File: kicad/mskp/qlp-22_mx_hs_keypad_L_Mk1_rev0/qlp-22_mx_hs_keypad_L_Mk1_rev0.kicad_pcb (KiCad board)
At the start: 2 copper layers, 175.4 x 84.9 mm, 28 parts, among them J1 Conn_01x12_Socket, SW0 Switch, SW1 Switch, SW10 Switch, SW2 Switch, SW3 Switch, SW4 Switch, SW5 Switch, SW6 Switch, SW7 Switch, SW8 Switch, SW9 Switch

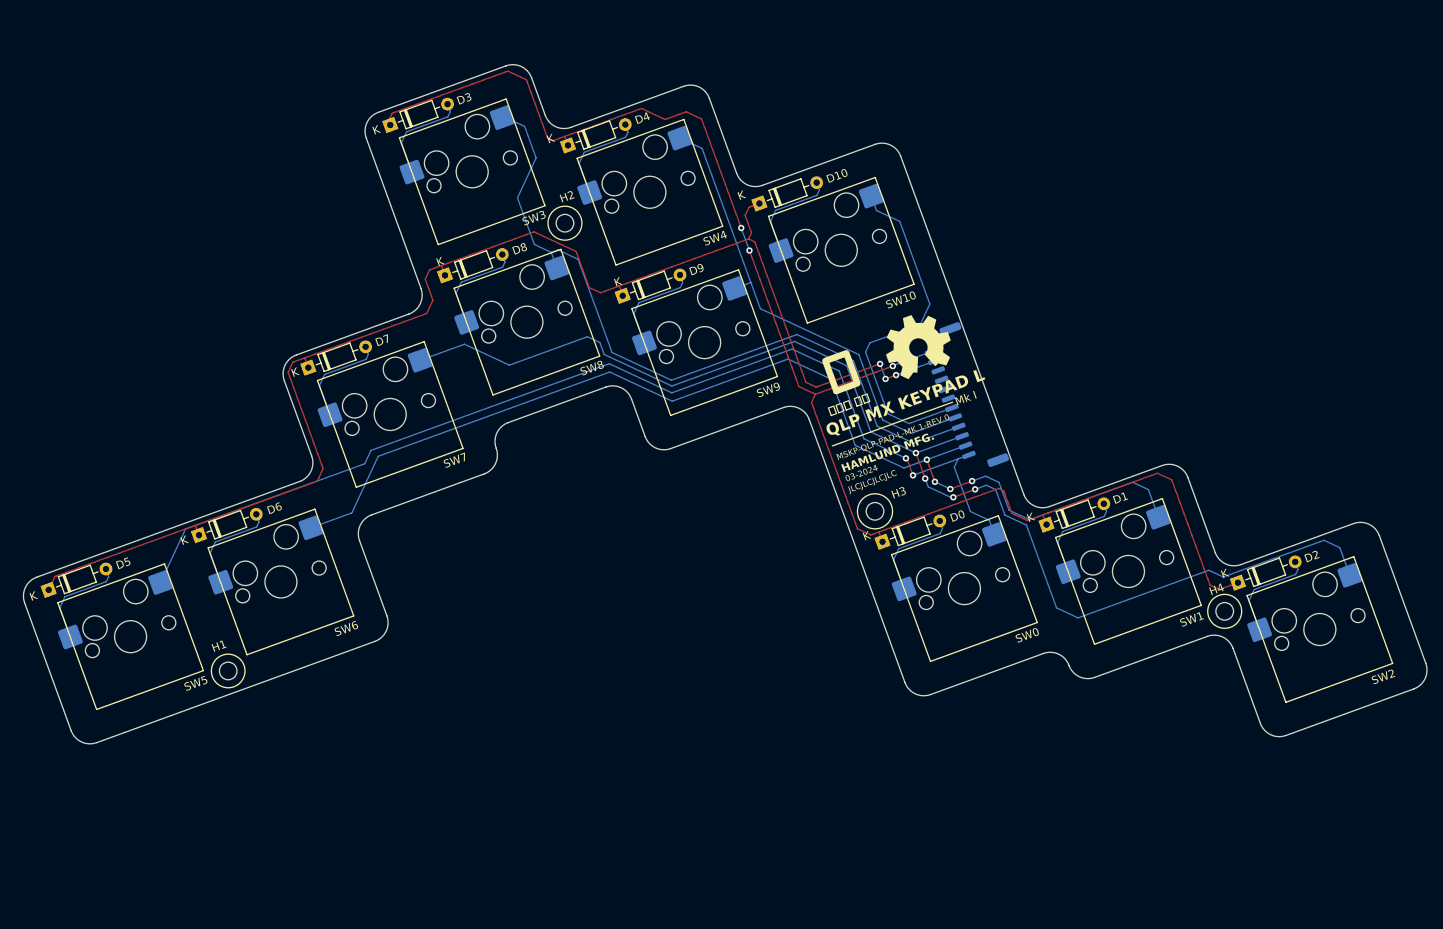
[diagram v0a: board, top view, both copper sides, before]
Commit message: Minor keypad design update ideas
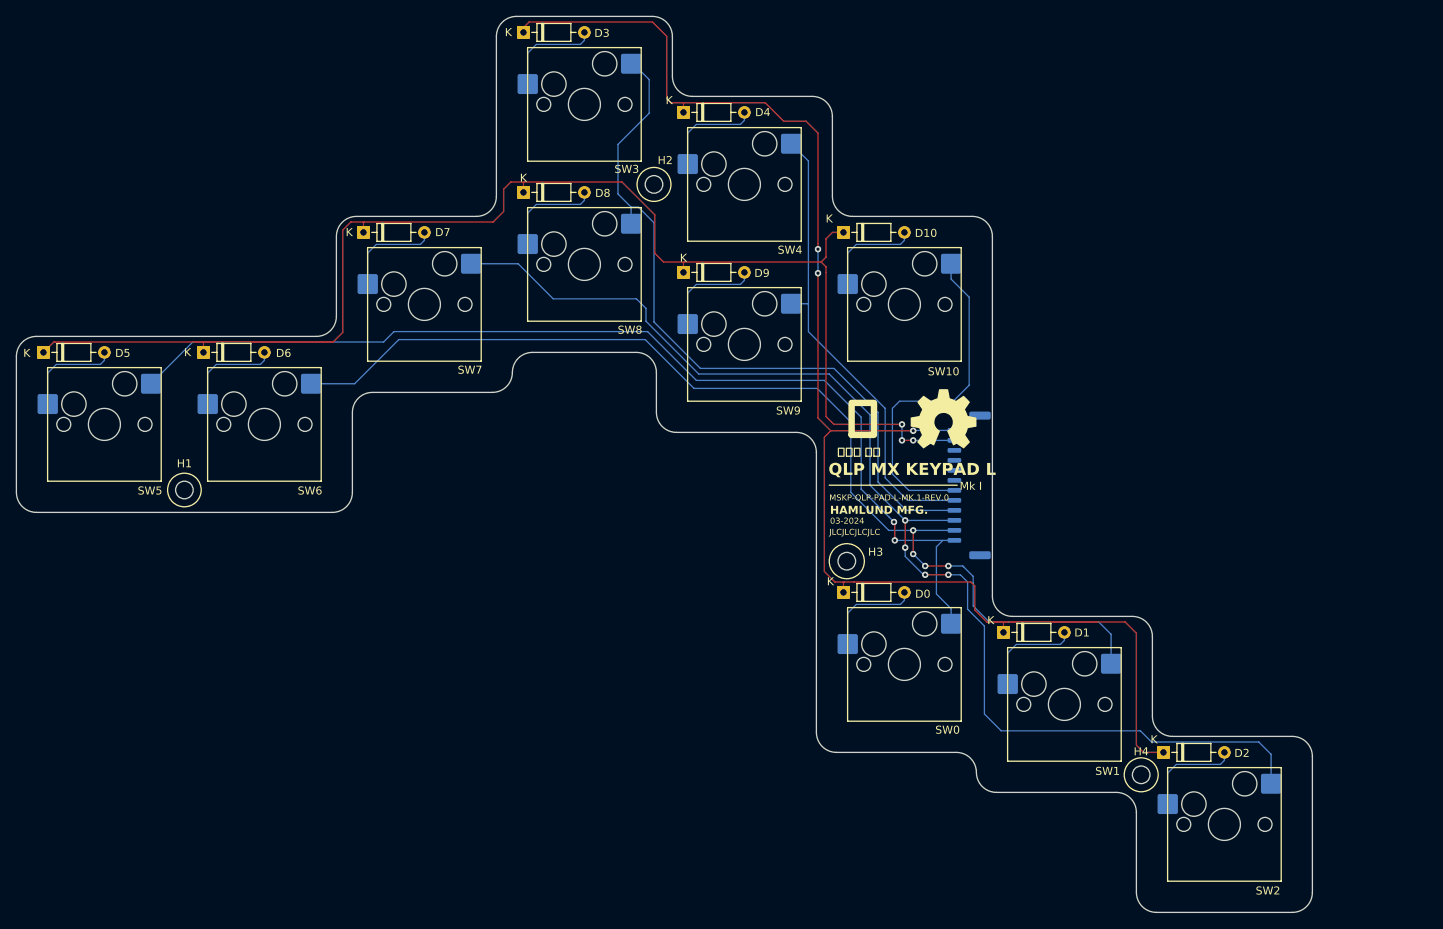
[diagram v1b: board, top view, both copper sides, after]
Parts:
- moved D5 29.7 mm to (57.0, 84.3), turned to 0 degrees
- moved SW2 27.1 mm to (204.6, 143.3), turned to 0 degrees
- moved SW5 26.7 mm to (64.6, 93.3), turned to 0 degrees
- moved H1 23.3 mm to (74.6, 101.5), turned to 0 degrees
- moved D2 23.2 mm to (197.0, 134.3), turned to 0 degrees
- moved H4 22.9 mm to (194.2, 137.1), turned to 0 degrees
- moved D6 22.9 mm to (77.0, 84.3), turned to 0 degrees
- moved D3 20.3 mm to (117.0, 44.3), turned to 0 degrees
- moved SW6 19.8 mm to (84.6, 93.3), turned to 0 degrees
- moved SW1 18.4 mm to (184.6, 128.3), turned to 0 degrees
- moved D7 18.3 mm to (97.0, 69.3), turned to 0 degrees
- moved SW3 16.4 mm to (124.6, 53.3), turned to 0 degrees
- moved D4 15.0 mm to (137.0, 54.3), turned to 0 degrees
- moved D1 14.5 mm to (177.0, 119.3), turned to 0 degrees
- moved SW7 14.4 mm to (104.6, 78.3), turned to 0 degrees
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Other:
- board size 175.4 x 84.9 mm -> 162 x 112 mm
